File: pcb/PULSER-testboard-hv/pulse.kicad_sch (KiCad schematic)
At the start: 21 parts, among them J1 Screw_Terminal 2pin, J2 Screw_Terminal 2pin, J3 Conn_01x02_Pin, J4 Conn_01x02_Pin, Q1 N-ch, Vds>=60V, fast switch, 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, U1 INA281A2, U10 LM317_DPAK, U2 LTC7001, U3 TL783, U7 TLV3201

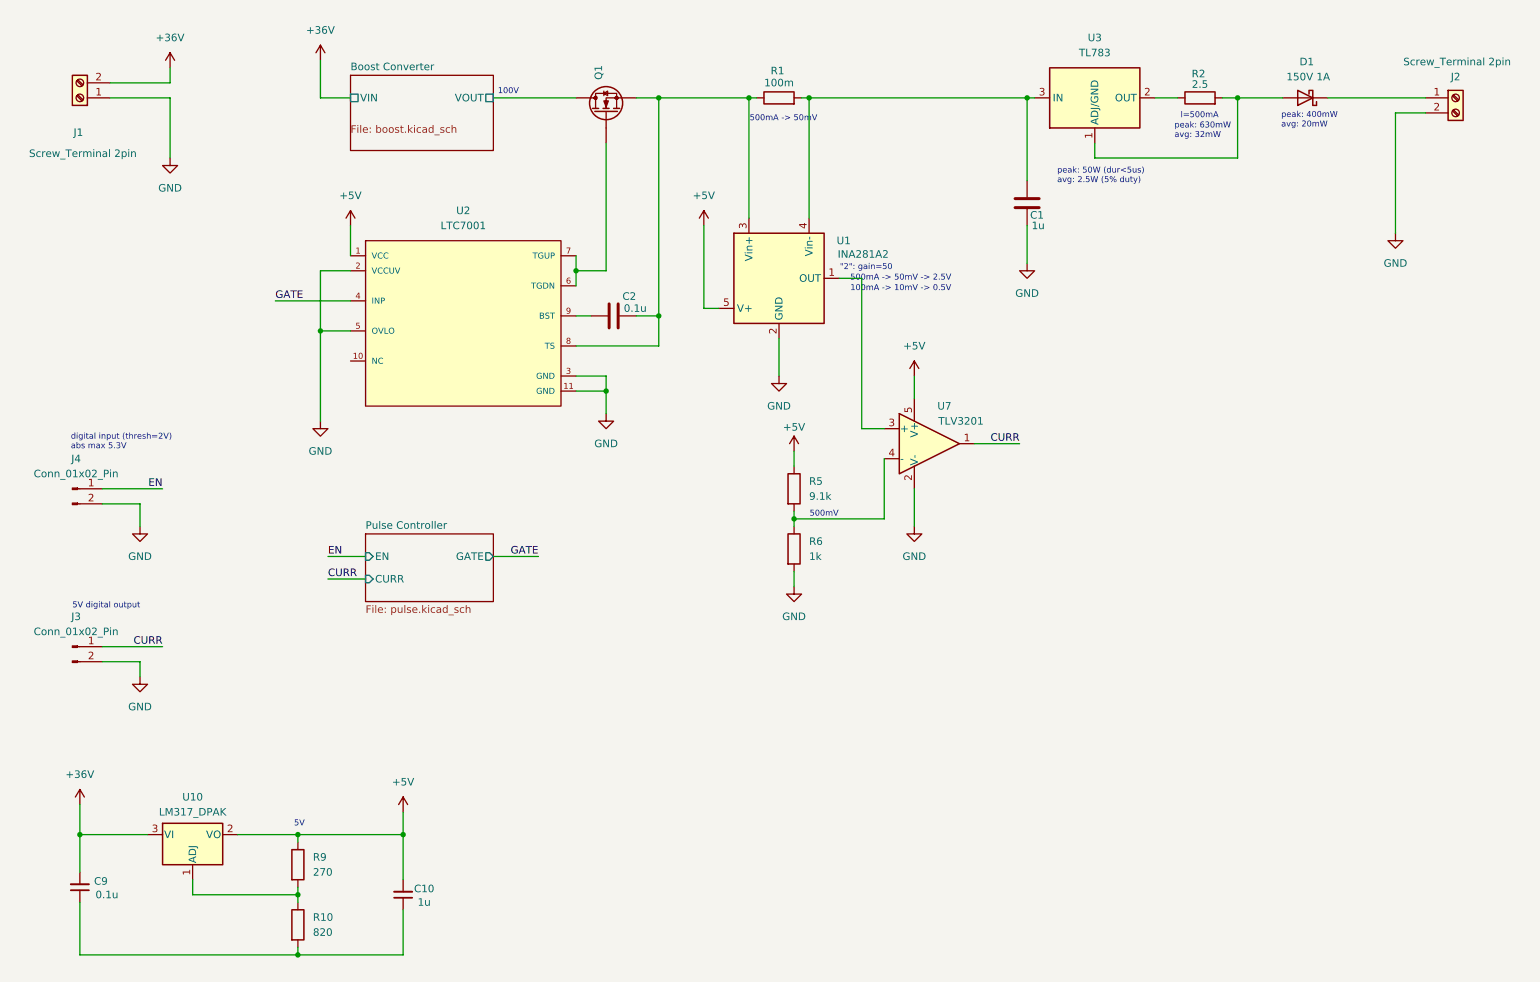
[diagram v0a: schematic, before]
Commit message: Draft architecture for both HC & HV
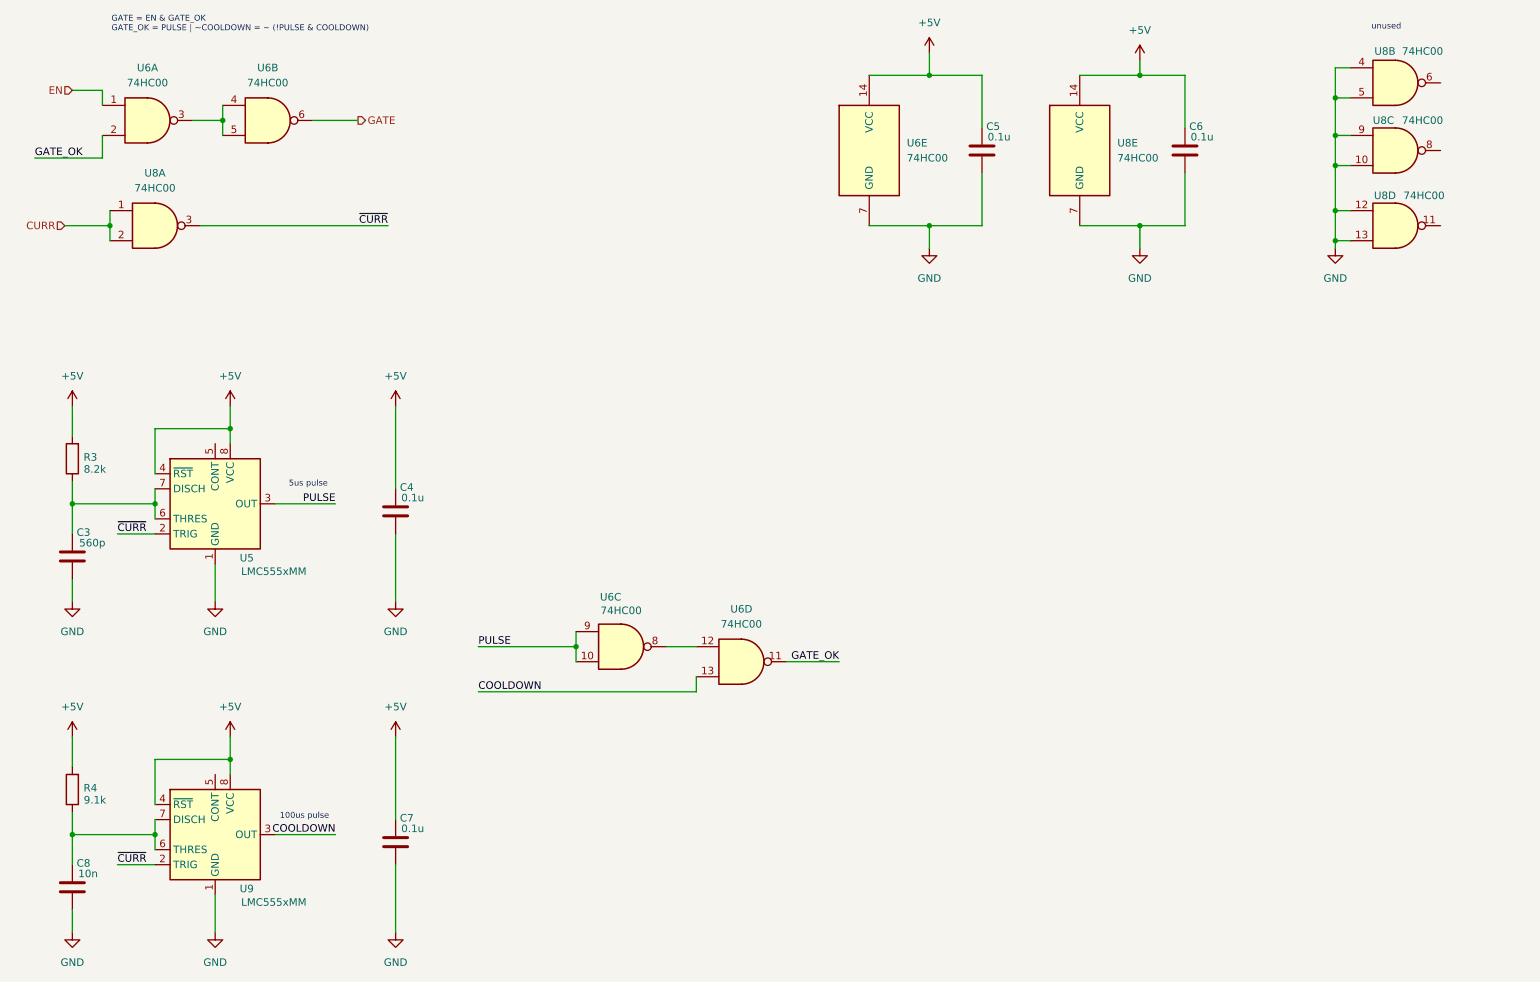
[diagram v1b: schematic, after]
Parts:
- removed C1: 1u, Capacitor_SMD:C_0603_1608Metric, symbol Device:C
- removed C10: 1u, symbol Device:C_Small
- removed C2: 0.1u, Capacitor_SMD:C_0603_1608Metric, symbol Device:C
- removed C9: 0.1u, symbol Device:C_Small
- removed D1: 150V 1A, Diode_SMD:D_PowerDI-123, symbol Device:D_Schottky
- removed J1, J2: Screw_Terminal 2pin, SparkAll:Wurth_TerminalBlock_2pin_P5mm_691137710002, symbol Connector:Screw_Terminal_01x02
- removed J3, J4: Conn_01x02_Pin, symbol Connector:Conn_01x02_Pin
- removed Q1: N-ch, Vds>=60V, fast switch, low Rds, SparkAll:Infineon-TG-TDSON-8-NMOS, symbol Device:Q_NMOS
- removed R1: 100m, Resistor_SMD:R_0603_1608Metric, symbol Device:R
- removed R10: 820, symbol Device:R
- removed R2: 2.5, Resistor_SMD:R_0603_1608Metric, symbol Device:R
- removed R5: 9.1k, symbol Device:R
- removed R6: 1k, symbol Device:R
- removed R9: 270, symbol Device:R
- removed U1: INA281A2, Package_TO_SOT_SMD:SOT-23-5, symbol Amplifier_Current:INA281A2
- removed U10: LM317_DPAK, Package_TO_SOT_SMD:TO-252-2, symbol Regulator_Linear:LM317_TO-252
- removed U2: LTC7001, Analog_Devices-MSE-10-05-08-1664-0-I-*, symbol SparkAll:LTC7001
- removed U3: TL783, Package_TO_SOT_SMD:TO-263-3_TabPin2, symbol Regulator_Linear:LD1086D2MTR
- removed U7: TLV3201, Package_TO_SOT_SMD:SOT-23-5, symbol Comparator:TLV7031DBV
- added C3: 560p, Capacitor_SMD:C_0603_1608Metric, symbol Device:C
- added C4, C5, C6, C7: 0.1u, Capacitor_SMD:C_0603_1608Metric, symbol Device:C
- added C8: 10n, Capacitor_SMD:C_0603_1608Metric, symbol Device:C
- added R3: 8.2k, Resistor_SMD:R_0603_1608Metric, symbol Device:R
- added R4: 9.1k, Resistor_SMD:R_0603_1608Metric, symbol Device:R
- added U5, U9: LMC555xMM, Package_SO:VSSOP-8_3x3mm_P0.65mm, symbol Timer:LMC555xMM
- added U6, U8: 74HC00, symbol 74xx:74HC00
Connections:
- net +5V: now also C4.2, C5.2, C6.2, C7.2, R3.2, R4.2, U5.4 (~{RST}), U5.8 (VCC), U6.14 (VCC), U8.14 (VCC), U9.4 (~{RST}), U9.8 (VCC)
- net CURR: now also U8.1, U8.2
- net EN: now also U6.1
- net GATE: now also U6.6
- net GND: now also C3.1, C4.1, C5.1, C6.1, C7.1, C8.1, U5.1 (GND), U6.7 (GND), U8.10, U8.12, U8.13, U8.4, U8.5, U8.7 (GND), U8.9, U9.1 (GND)
- new net: C8.2, R4.1, U9.6 (THRES), U9.7 (DISCH)
- new net: U6.12, U6.8
- new net: C3.2, R3.1, U5.6 (THRES), U5.7 (DISCH)
- new net: U6.3, U6.4, U6.5
- new net COOLDOWN: U6.13, U9.3 (OUT)
- new net GATE_OK: U6.11, U6.2
- new net PULSE: U5.3 (OUT), U6.10, U6.9
- new net ~{CURR}: U5.2 (TRIG), U8.3, U9.2 (TRIG)
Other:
- removed sheet Boost Converter
- removed sheet Pulse Controller
- note added: "100us pulse"
- note added: "5us pulse"
- note added: "GATE = EN & GATE_OK GATE_OK = PULSE | ~COOLDOWN = ~ (!PULSE & COOLDOWN)"
- note added: "unused"
- note removed: ""2": gain=50"
- note removed: "100V"
- note removed: "100mA -> 10mV -> 0.5V"
- note removed: "500mA -> 50mV"
- note removed: "500mA -> 50mV -> 2.5V"
- note removed: "500mV"
- note removed: "5V"
- note removed: "5V digital output"
- note removed: "I=500mA"
- note removed: "digital input (thresh=2V) abs max 5.3V"
- note removed: "peak: 400mW avg: 20mW"
- note removed: "peak: 50W (dur<5us) avg: 2.5W (5% duty)"
- note removed: "peak: 630mW avg: 32mW"
